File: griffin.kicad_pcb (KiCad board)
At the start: 2 copper layers, 150 x 100 mm, 43 parts, among them IC1 ME6211C33M5G-N, J1 USB_B_Micro, J2 Conn_02x03_Odd_Even, J3 Conn_01x04, J4 Conn_01x11, J5 Conn_01x04, J6 Conn_01x20, J7 Conn_01x20, J8 Conn_01x14, J9 Conn_01x08, P1 USB_C_Plug, SW1 SW_Push, SW2 SW_Push, SW3 SW_Push, U1 STM32F103C8Tx, Y1 32.768KHz, Y2 8MHz

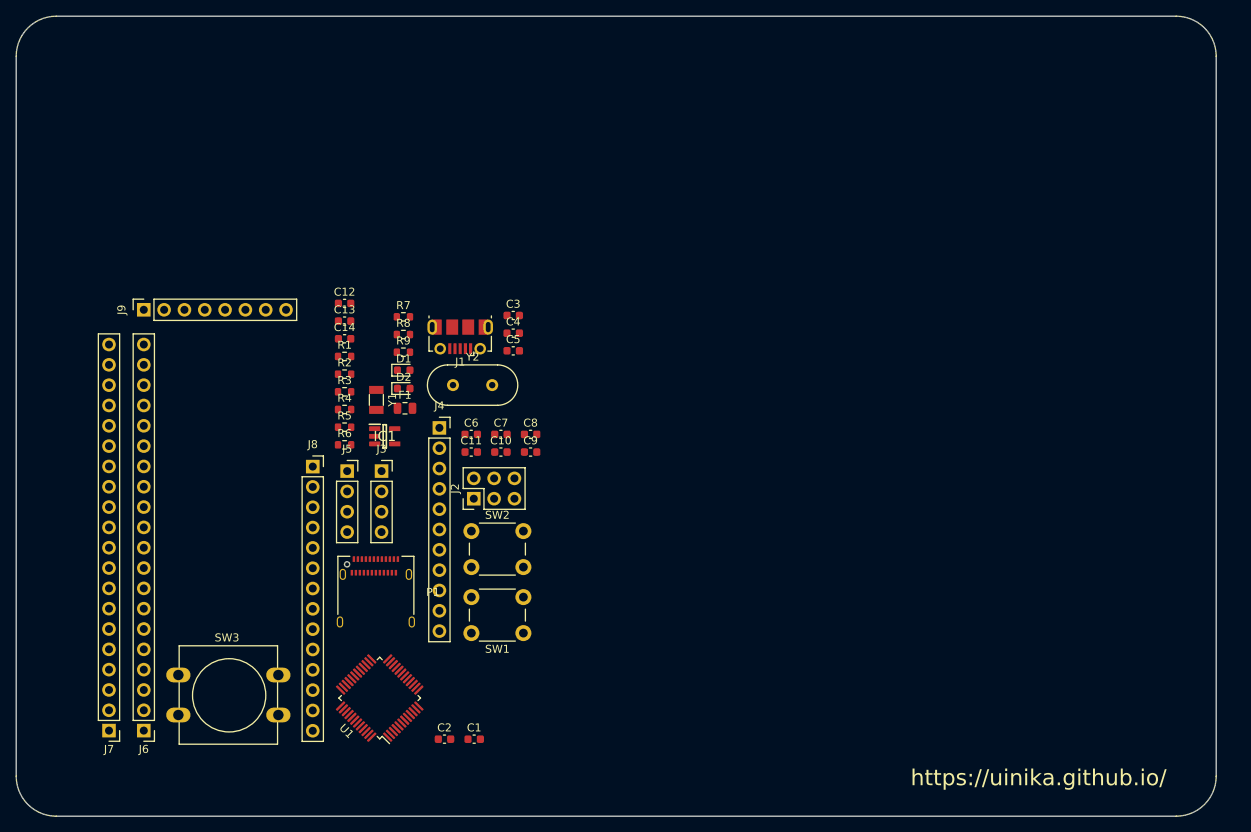
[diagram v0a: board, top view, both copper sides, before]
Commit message: update PCB
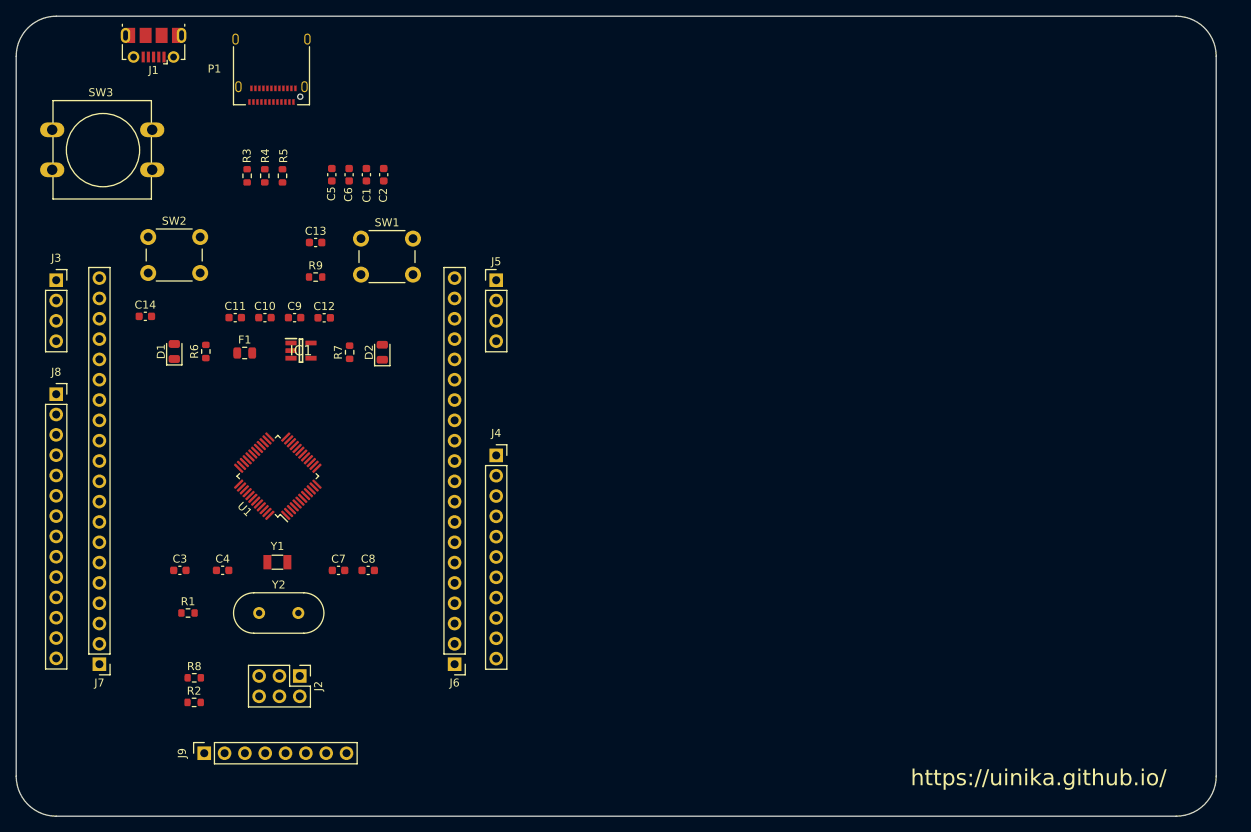
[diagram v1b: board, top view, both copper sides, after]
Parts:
- D1: value LED -> LED1; footprint LED_SMD:LED_0603_1608Metric -> LED_SMD:LED_0805_2012Metric
- D2: value LED -> LED2; footprint LED_SMD:LED_0603_1608Metric -> LED_SMD:LED_0805_2012Metric
- J5: footprint Connector_PinSocket_2.54mm:PinSocket_1x04_P2.54mm_Vertical -> Connector_PinHeader_2.54mm:PinHeader_1x04_P2.54mm_Vertical
- moved C1 71.8 mm to (85.8, 60.8), turned to 270 degrees
- moved C2 71.0 mm to (87.9, 60.8), turned to 270 degrees
- moved SW3 70.0 mm to (46.5, 55.2)
- moved P1 68.4 mm to (73.9, 46.7), turned to 180 degrees
- moved J9 55.9 mm to (65.5, 133.1)
- moved SW2 54.6 mm to (58.5, 68.6)
- moved SW1 53.3 mm to (85.1, 68.8), turned to 0 degrees
- moved J1 52.9 mm to (59.2, 44.6)
- moved C3 52.5 mm to (62.5, 110.3)
- moved R8 50.2 mm to (64.3, 123.7)
- moved J3 47.2 mm to (47.0, 74.0)
- moved C4 46.9 mm to (67.8, 110.3)
- moved R2 45.1 mm to (64.2, 126.8)
- moved J6 39.7 mm to (96.8, 122.0)
- moved R1 37.6 mm to (63.5, 115.6)
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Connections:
- net /+5V renamed +5V
- R7 pad 2: GND -> /LED2
